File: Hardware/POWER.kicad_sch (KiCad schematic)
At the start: 65 parts, among them J15 5V_USB, J17 Battery IN, Q1 RE1C002UN, U11 AOZ1212AI, U5 AP2112K-3.3, U5 AP2151W, U6 AP2112K-1.8, U7 AP2112K-3.3

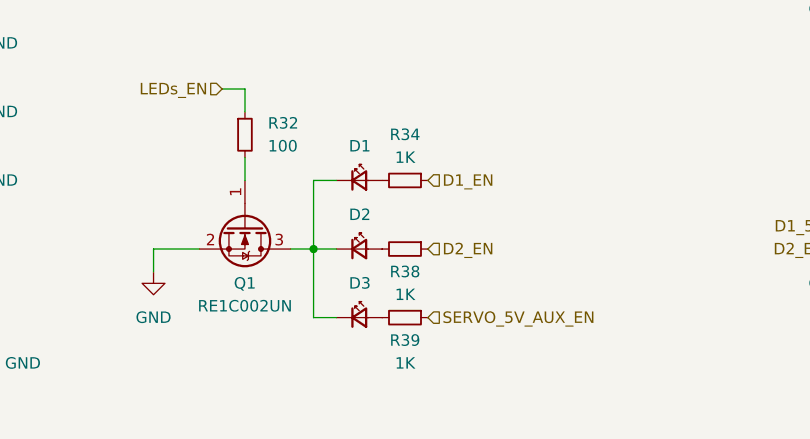
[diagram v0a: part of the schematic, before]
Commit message: Checkpoint
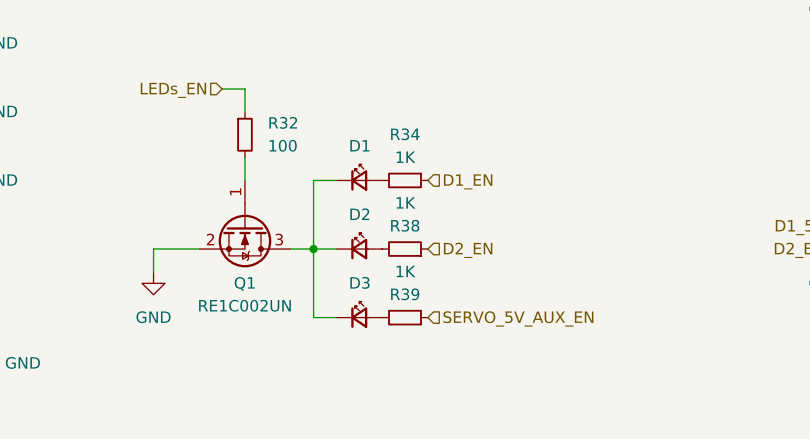
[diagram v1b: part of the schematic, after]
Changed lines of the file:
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@@
     )
   )
-  (symbol (lib_id "Device:R_Small") (at 93.98 185.42 270) (unit 1)
-    (in_bom yes) (on_board yes) (dnp no) (fields_autoplaced)
-    (property "Reference" "R39" (at 93.98 187.96 90)
-      (effects (font (size 1.27 1.27)))
-    )
-    (property "Value" "1K" (at 93.98 190.5 90)
+  (symbol (lib_id "Device:R_Small") (at 93.98 185.42 270) (mirror x) (unit 1)
+    (in_bom yes) (on_board yes) (dnp no)
+    (property "Reference" "R39" (at 93.98 182.88 90)
+      (effects (font (size 1.27 1.27)))
+    )
+    (property "Value" "1K" (at 93.98 180.34 90)
       (effects (font (size 1.27 1.27)))
     )
@@
     )
   )
-  (symbol (lib_id "Device:R_Small") (at 93.98 177.8 270) (unit 1)
-    (in_bom yes) (on_board yes) (dnp no) (fields_autoplaced)
-    (property "Reference" "R38" (at 93.98 180.34 90)
-      (effects (font (size 1.27 1.27)))
-    )
-    (property "Value" "1K" (at 93.98 182.88 90)
+  (symbol (lib_id "Device:R_Small") (at 93.98 177.8 270) (mirror x) (unit 1)
+    (in_bom yes) (on_board yes) (dnp no)
+    (property "Reference" "R38" (at 93.98 175.26 90)
+      (effects (font (size 1.27 1.27)))
+    )
+    (property "Value" "1K" (at 93.98 172.72 90)
       (effects (font (size 1.27 1.27)))
     )
@@
   )
   (symbol (lib_id "Device:R_Small") (at 93.98 170.18 270) (unit 1)
-    (in_bom yes) (on_board yes) (dnp no) (fields_autoplaced)
+    (in_bom yes) (on_board yes) (dnp no)
     (property "Reference" "R34" (at 93.98 165.1 90)
       (effects (font (size 1.27 1.27)))
